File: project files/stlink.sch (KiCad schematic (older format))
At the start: 57 parts, among them J1 USB_C_Receptacle_USB2.0, J2 SELF, J3 SWD, J4 TARGET, Q1 MMBT9013, U1 STM32F103CBTx, U2 AMS1117-3.3, Y1 8MHz

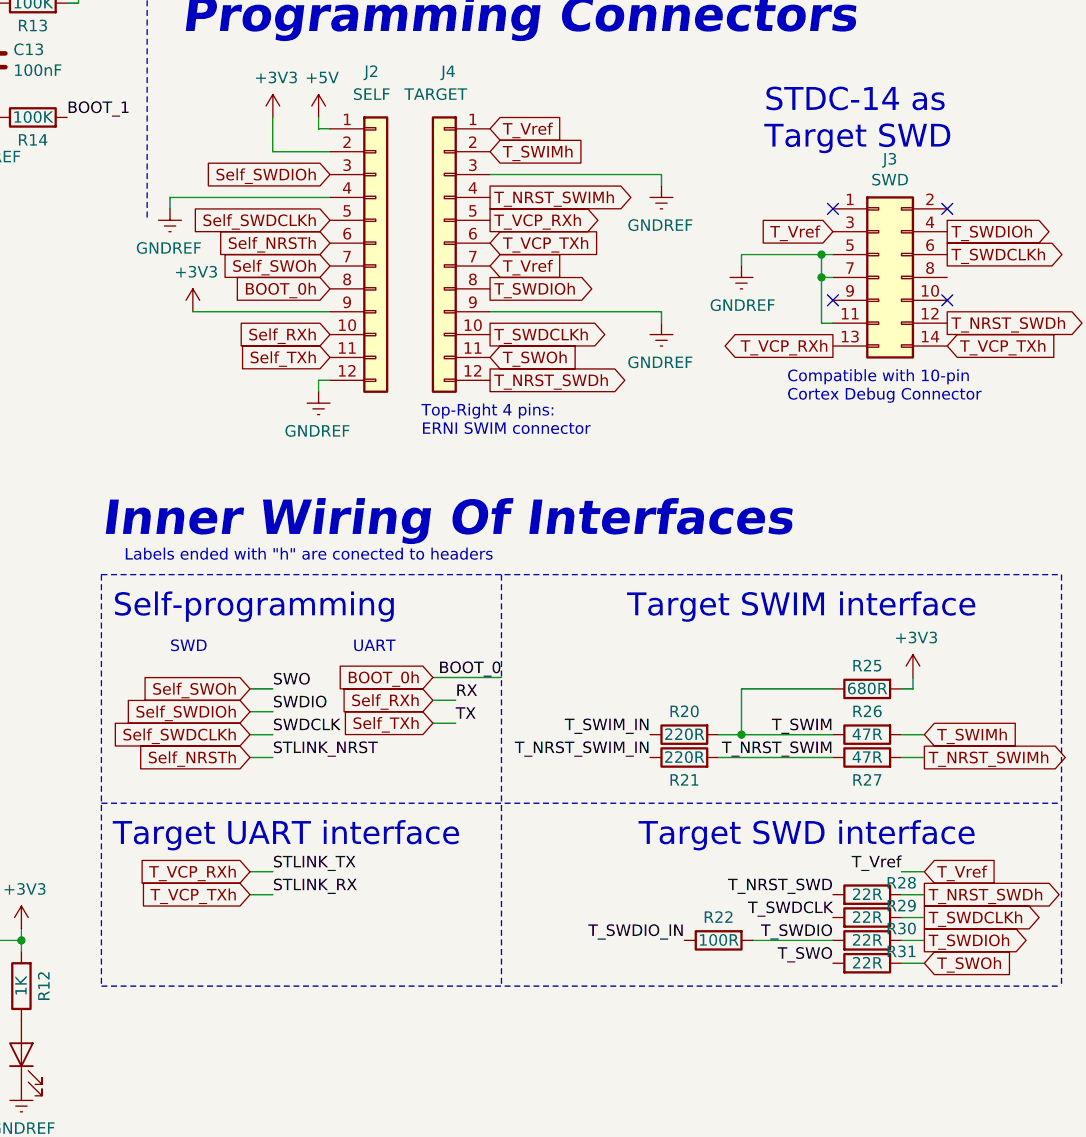
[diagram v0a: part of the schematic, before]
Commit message: ajfdlsa;jd;sakd
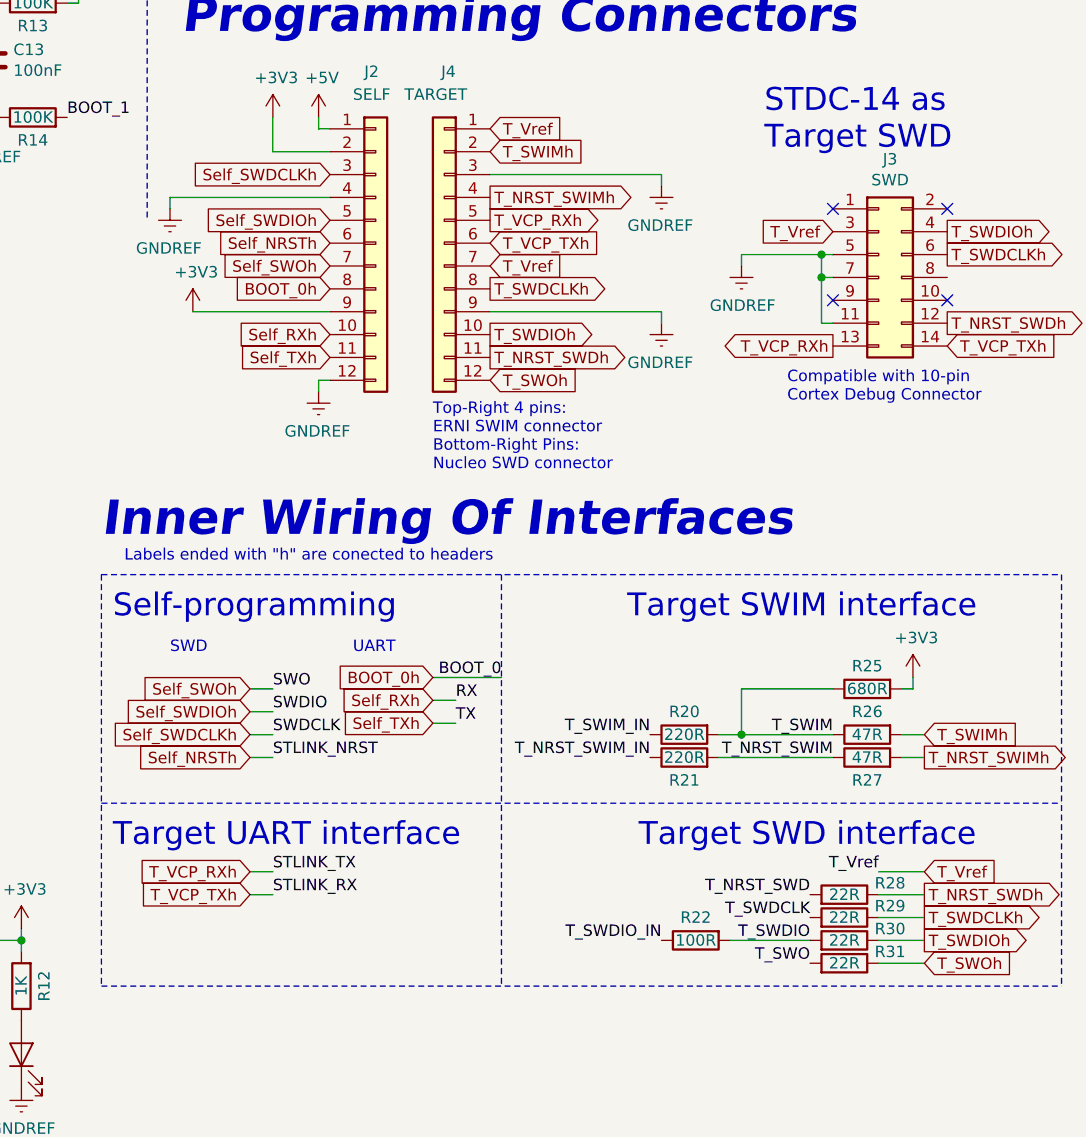
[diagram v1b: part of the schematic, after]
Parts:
- F1: footprint Fuse:Fuse_1210_3225Metric -> Fuse:Fuse_1206_3216Metric
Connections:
- net Self_SWDCLKh: now also J2.3 (Pin_3); no longer J2.5 (Pin_5)
- net Self_SWDIOh: now also J2.5 (Pin_5); no longer J2.3 (Pin_3)
- net T_NRST_SWDh: now also J4.11 (Pin_11); no longer J4.12 (Pin_12)
- net T_SWDCLKh: now also J4.8 (Pin_8); no longer J4.10 (Pin_10)
- net T_SWDIOh: now also J4.10 (Pin_10); no longer J4.8 (Pin_8)
- net T_SWOh: now also J4.12 (Pin_12); no longer J4.11 (Pin_11)
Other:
- note added: "Top-Right 4 pins:\nERNI SWIM connector\nBottom-Right Pins: \nNucleo SWD connector"
- note removed: "Top-Right 4 pins:\nERNI SWIM connector"
- moved on the sheet: R22, R28, R29, R30, R31
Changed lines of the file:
@@
 Text Label 10200 5500 2    50   ~ 0
 T_NRST_SWIM
-Wire Wire Line
-	10600 6400 10500 6400
-Wire Wire Line
-	10600 6300 10500 6300
-Wire Wire Line
-	10600 6200 10500 6200
-Wire Wire Line
-	10600 6100 10500 6100
-Wire Wire Line
-	10600 6000 10500 6000
-Text Label 10200 6400 2    50   ~ 0
+Text Label 10100 6400 2    50   ~ 0
 T_SWO
-Text Label 10200 6300 2    50   ~ 0
+Text Label 10100 6300 2    50   ~ 0
 T_SWDIO
-Text Label 10200 6200 2    50   ~ 0
+Text Label 10100 6200 2    50   ~ 0
 T_SWDCLK
-Text Label 10200 6100 2    50   ~ 0
+Text Label 10100 6100 2    50   ~ 0
 T_NRST_SWD
-Text Label 10500 6000 2    50   ~ 0
+Text Label 10400 6000 2    50   ~ 0
 T_Vref
 NoConn ~ 1150 5550
@@
 NoConn ~ 1150 5250
 $Comp
-L Device:R R31
-U 1 1 5E239BA0
-P 10350 6400
-F 0 "R31" V 10400 6550 50  0000 C CNN
-F 1 "22R" V 10350 6400 50  0000 C CNN
-F 2 "Resistor_SMD:R_0603_1608Metric_Pad1.05x0.95mm_HandSolder" V 10280 6400 50  0001 C CNN
-F 3 "~" H 10350 6400 50  0001 C CNN
-	1    10350 6400
-	0    1    -1   0
-$EndComp
-$Comp
-L Device:R R30
-U 1 1 5E241EAA
-P 10350 6300
-F 0 "R30" V 10400 6450 50  0000 C CNN
-F 1 "22R" V 10350 6300 50  0000 C CNN
-F 2 "Resistor_SMD:R_0603_1608Metric_Pad1.05x0.95mm_HandSolder" V 10280 6300 50  0001 C CNN
-F 3 "~" H 10350 6300 50  0001 C CNN
-	1    10350 6300
-	0    1    -1   0
-$EndComp
-$Comp
 L Device:R R29
 U 1 1 5E241FEE
-P 10350 6200
-F 0 "R29" V 10400 6350 50  0000 C CNN
-F 1 "22R" V 10350 6200 50  0000 C CNN
-F 2 "Resistor_SMD:R_0603_1608Metric_Pad1.05x0.95mm_HandSolder" V 10280 6200 50  0001 C CNN
-F 3 "~" H 10350 6200 50  0001 C CNN
-	1    10350 6200
+P 10250 6200
+F 0 "R29" V 10300 6400 50  0000 C CNN
+F 1 "22R" V 10250 6200 50  0000 C CNN
+F 2 "Resistor_SMD:R_0603_1608Metric_Pad1.05x0.95mm_HandSolder" V 10180 6200 50  0001 C CNN
+F 3 "~" H 10250 6200 50  0001 C CNN
+	1    10250 6200
 	0    1    -1   0
 $EndComp
@@
 L Device:R R28
 U 1 1 5E242103
-P 10350 6100
-F 0 "R28" V 10400 6250 50  0000 C CNN
-F 1 "22R" V 10350 6100 50  0000 C CNN
-F 2 "Resistor_SMD:R_0603_1608Metric_Pad1.05x0.95mm_HandSolder" V 10280 6100 50  0001 C CNN
-F 3 "~" H 10350 6100 50  0001 C CNN
-	1    10350 6100
+P 10250 6100
+F 0 "R28" V 10300 6300 50  0000 C CNN
+F 1 "22R" V 10250 6100 50  0000 C CNN
+F 2 "Resistor_SMD:R_0603_1608Metric_Pad1.05x0.95mm_HandSolder" V 10180 6100 50  0001 C CNN
+F 3 "~" H 10250 6100 50  0001 C CNN
+	1    10250 6100
 	0    1    -1   0
 $EndComp
@@
 L Device:R R22
 U 1 1 5E2426E2
-P 9700 6300
-F 0 "R22" V 9600 6300 50  0000 C CNN
-F 1 "100R" V 9700 6300 50  0000 C CNN
-F 2 "Resistor_SMD:R_0603_1608Metric_Pad1.05x0.95mm_HandSolder" V 9630 6300 50  0001 C CNN
-F 3 "~" H 9700 6300 50  0001 C CNN
-	1    9700 6300
+P 9600 6300
+F 0 "R22" V 9500 6300 50  0000 C CNN
+F 1 "100R" V 9600 6300 50  0000 C CNN
+F 2 "Resistor_SMD:R_0603_1608Metric_Pad1.05x0.95mm_HandSolder" V 9530 6300 50  0001 C CNN
+F 3 "~" H 9600 6300 50  0001 C CNN
+	1    9600 6300
 	0    -1   1    0
 $EndComp
-Text Label 9550 6300 2    50   ~ 0
+Text Label 9450 6300 2    50   ~ 0
 T_SWDIO_IN
 Text Label 1150 6350 2    50   ~ 0
@@
 T_SWDIO
 Wire Wire Line
-	10200 6300 9850 6300
+	10100 6300 9750 6300
 Text Label 2450 5650 0    50   ~ 0
 T_SWDCLK
@@
 Text GLabel 10700 3300 2    50   Output ~ 0
 T_SWDCLKh
-Text GLabel 8700 3750 2    50   Input ~ 0
+Text GLabel 8700 3850 2    50   Input ~ 0
 T_SWOh
 Text GLabel 10700 3600 2    50   Output ~ 0
@@
 F 0 "F1" V 1575 1100 50  0000 C CNN
 F 1 "1A" V 1666 1100 50  0000 C CNN
-F 2 "Fuse:Fuse_1210_3225Metric" H 1850 900 50  0001 L CNN
+F 2 "Fuse:Fuse_1206_3216Metric" H 1850 900 50  0001 L CNN
 F 3 "~" H 1800 1100 50  0001 C CNN
 	1    1800 1100
@@
 Text GLabel 8700 3350 2    50   Input ~ 0
 T_Vref
-Text GLabel 8700 3450 2    50   Output ~ 0
+Text GLabel 8700 3650 2    50   Output ~ 0
 T_SWDIOh
 $Comp
@@
 	-1   0    0    -1
 $EndComp
-Text GLabel 8700 3650 2    50   Output ~ 0
+Text GLabel 8700 3450 2    50   Output ~ 0
 T_SWDCLKh
-Text GLabel 8700 3850 2    50   Output ~ 0
+Text GLabel 8700 3750 2    50   Output ~ 0
 T_NRST_SWDh
 Text GLabel 8700 3150 2    50   Output ~ 0
@@
 	1    0    0    -1
 $EndComp
-Text GLabel 8000 2950 0    50   Input ~ 0
+Text GLabel 8000 3150 0    50   Input ~ 0
 Self_SWDIOh
 $Comp
@@
 	-1   0    0    -1
 $EndComp
-Text GLabel 8000 3150 0    50   Input ~ 0
+Text GLabel 8000 2950 0    50   Input ~ 0
 Self_SWDCLKh
 Text GLabel 8000 3250 0    50   Input ~ 0
@@
 Wire Wire Line
 	7750 2850 7750 2700
-Text Notes 8400 4100 0    50   ~ 0
-Top-Right 4 pins:\nERNI SWIM connector
+Text Notes 8450 4250 0    50   ~ 0
+Top-Right 4 pins:\nERNI SWIM connector\nBottom-Right Pins: \nNucleo SWD connector
 Wire Wire Line
 	6550 2200 6500 2200
@@
 	-1   0    0    -1
 $EndComp
+$Comp
+L Device:R R30
+U 1 1 5E241EAA
+P 10250 6300
+F 0 "R30" V 10300 6500 50  0000 C CNN
+F 1 "22R" V 10250 6300 50  0000 C CNN
+F 2 "Resistor_SMD:R_0603_1608Metric_Pad1.05x0.95mm_HandSolder" V 10180 6300 50  0001 C CNN
+F 3 "~" H 10250 6300 50  0001 C CNN
+	1    10250 6300
+	0    1    -1   0
+$EndComp
+$Comp
+L Device:R R31
+U 1 1 5E239BA0
+P 10250 6400
+F 0 "R31" V 10300 6600 50  0000 C CNN
+F 1 "22R" V 10250 6400 50  0000 C CNN
+F 2 "Resistor_SMD:R_0603_1608Metric_Pad1.05x0.95mm_HandSolder" V 10180 6400 50  0001 C CNN
+F 3 "~" H 10250 6400 50  0001 C CNN
+	1    10250 6400
+	0    1    -1   0
+$EndComp
+Wire Wire Line
+	10400 6100 10600 6100
+Wire Wire Line
+	10400 6200 10600 6200
+Wire Wire Line
+	10400 6300 10600 6300
+Wire Wire Line
+	10400 6400 10600 6400
+Wire Wire Line
+	10400 6000 10600 6000
 $EndSCHEMATC
